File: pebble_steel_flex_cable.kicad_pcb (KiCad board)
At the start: 2 copper layers, 79.2 x 17.8 mm, 33 parts, among them CN1 5v, CN2 GND, J1 505551-1620, SW1 Select, SW2 UP, SW3 Down, SW4 Back, U1 IS31FL3199-QFLS2-TR

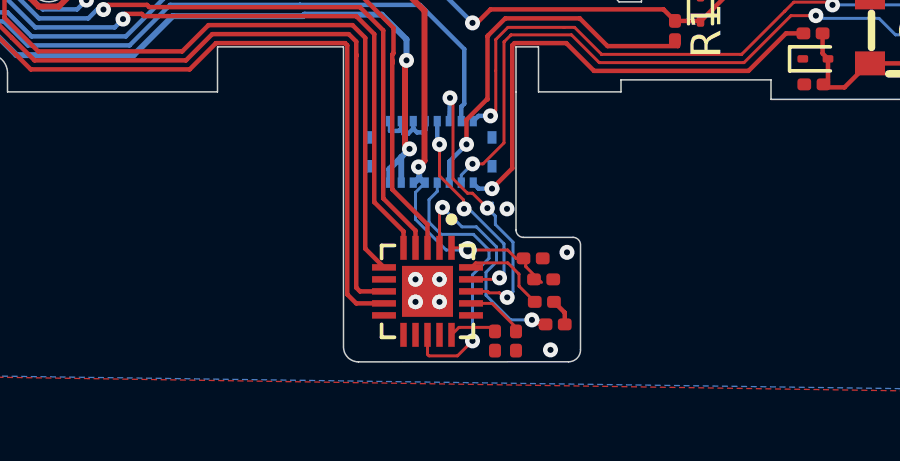
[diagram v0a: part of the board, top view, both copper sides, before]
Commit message: not sure what changed
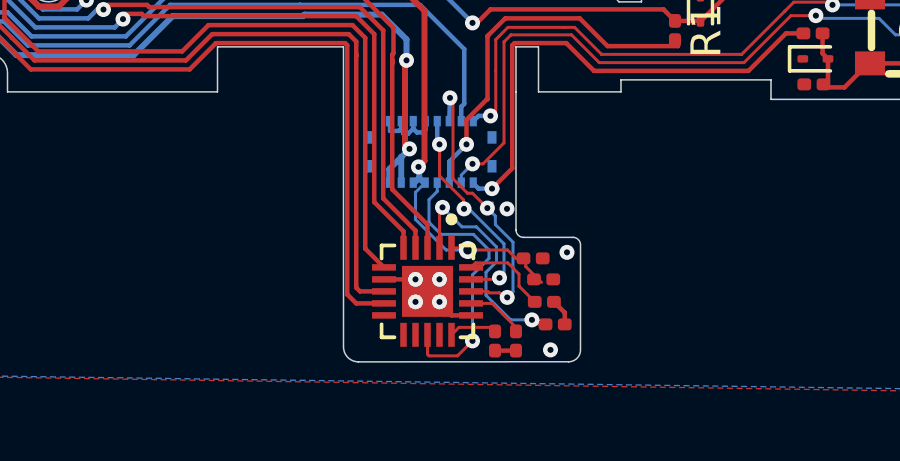
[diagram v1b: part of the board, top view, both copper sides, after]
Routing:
- net GND: track 3.53 -> 7.06 mm
